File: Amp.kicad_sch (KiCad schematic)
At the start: 37 parts, among them J1 Screw_Terminal_01x02, J2 AudioJack2, J3 Screw_Terminal_01x02, J4 Screw_Terminal_01x02, J5 Screw_Terminal_01x02, P1 100k, U1 ECC83, U2 EL34, U3 EL34

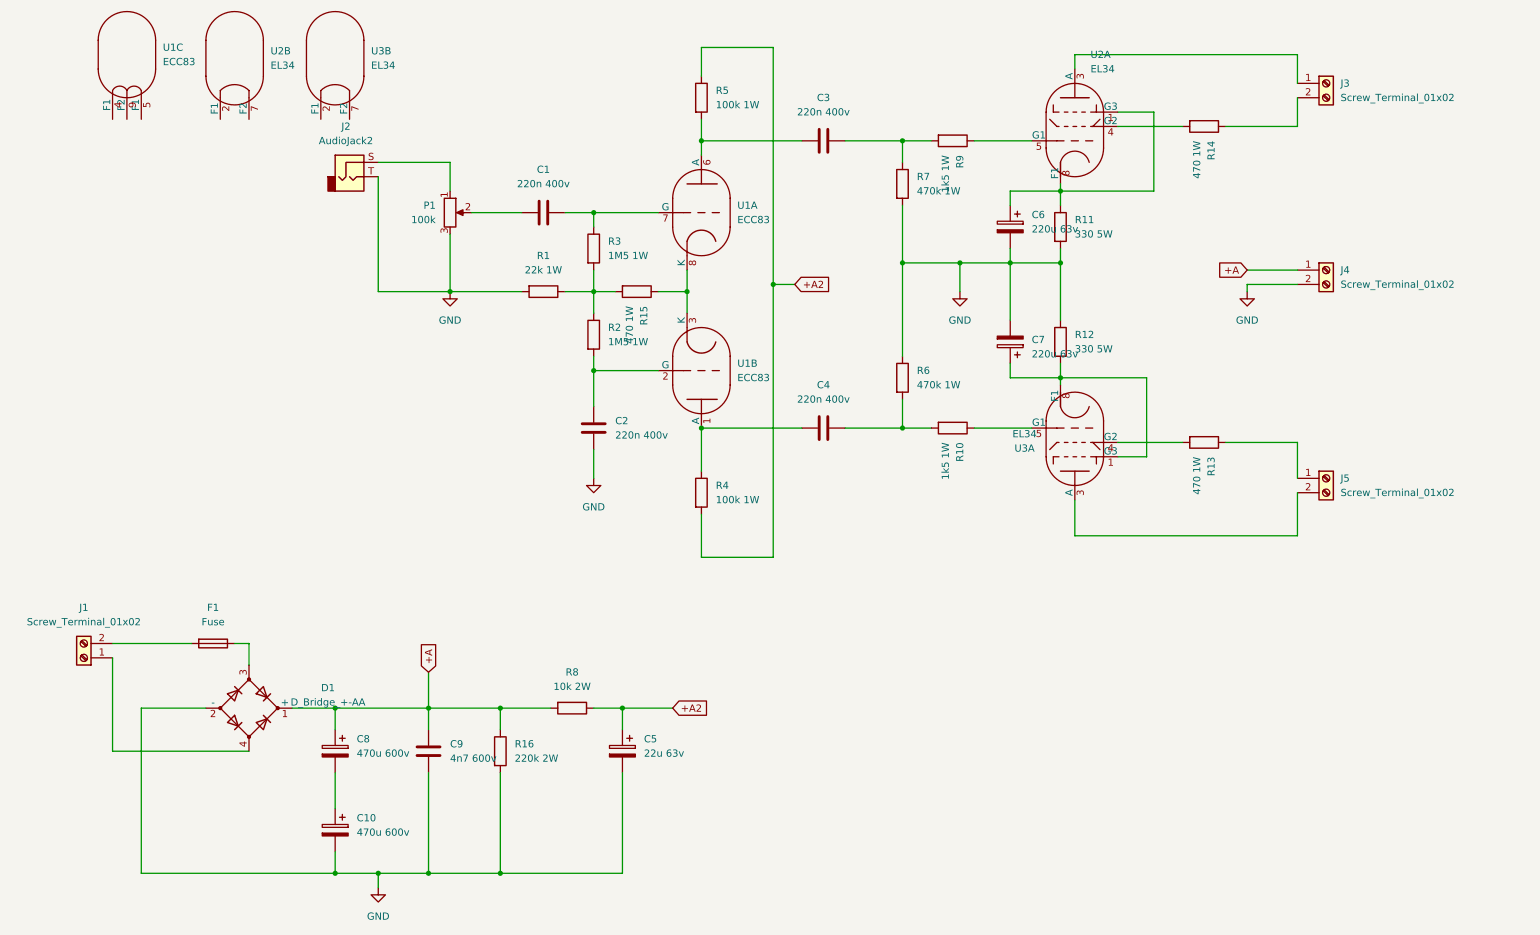
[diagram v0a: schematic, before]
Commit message: Update
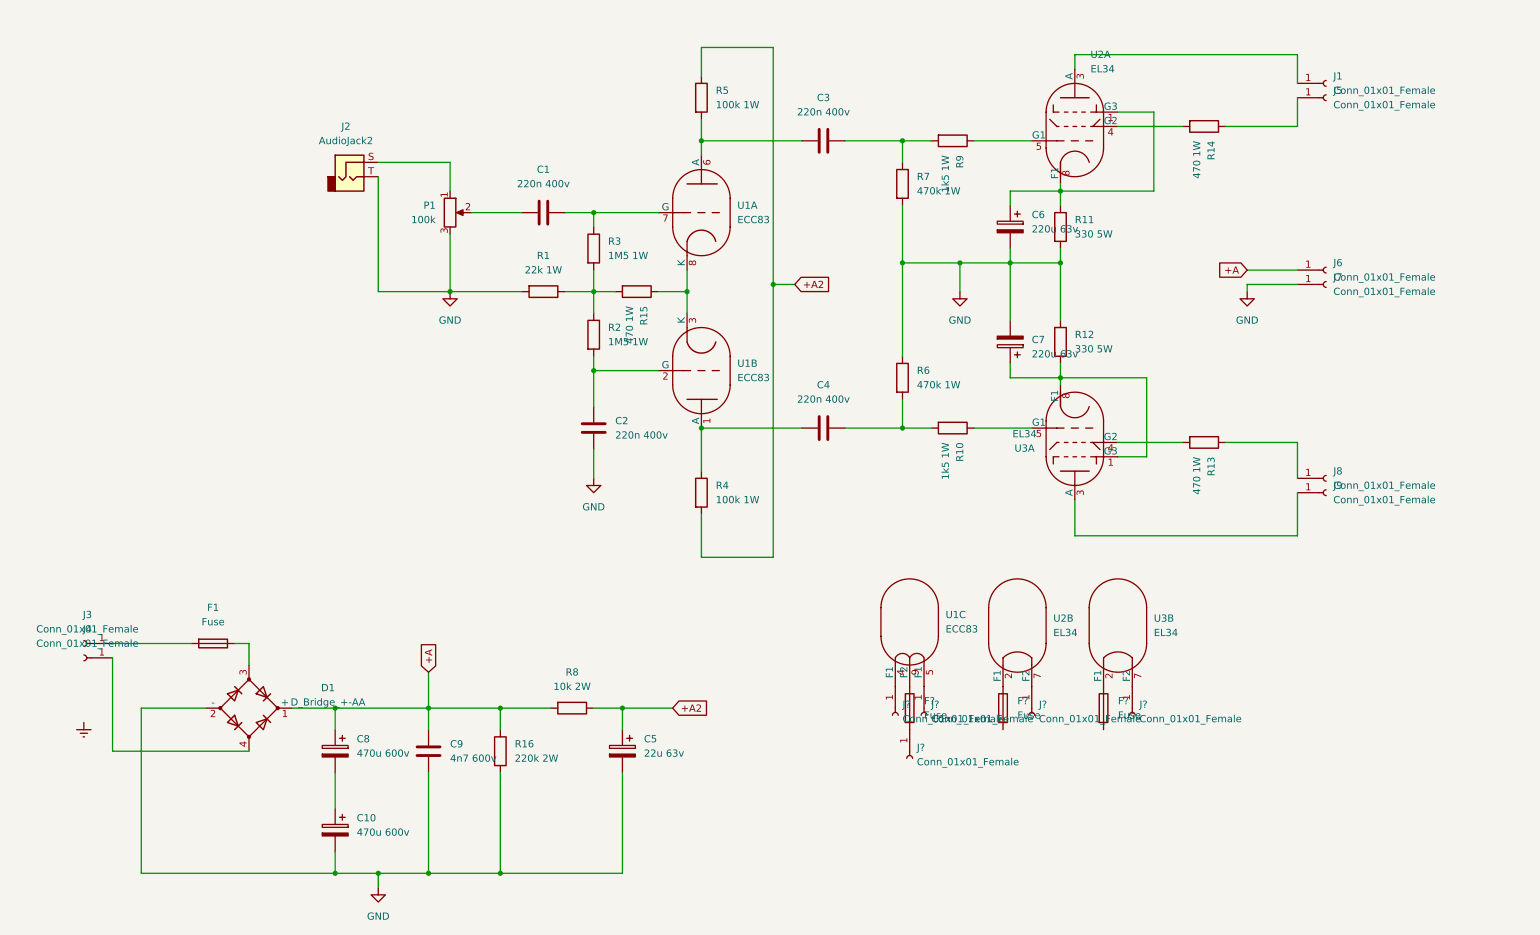
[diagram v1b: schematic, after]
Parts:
- removed J1, J3, J4, J5: Screw_Terminal_01x02, Connector:Banana_Jack_2Pin, symbol Connector:Screw_Terminal_01x02
- added F? (x3): Fuse, Fuse:Fuseholder_Cylinder-5x20mm_Schurter_0031_8201_Horizontal_Open, symbol Device:Fuse
- added J1, J3, J4, J5, J6, J7, J8, J9, J? (x5): Conn_01x01_Female, Connector_Pin:Pin_D1.0mm_L10.0mm, symbol Connector:Conn_01x01_Female
- F1: footprint (none) -> Fuse:Fuseholder_Cylinder-5x20mm_Schurter_0031_8201_Horizontal_Open
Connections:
- net +A: now also J6.1 (Pin_1)
- net GND: now also J7.1 (Pin_1)
- net at D1.4: now also J4.1 (Pin_1)
- net at F1.2: now also J3.1 (Pin_1)
- net at U1.4 (F1): now also J?.1 (Pin_1)
- net at U1.5 (F1): now also J?.1 (Pin_1)
- net at U1.9 (F2): now also F?.1
- net at R14.1: now also J5.1 (Pin_1)
- net at R13.1: now also J8.1 (Pin_1)
- net at U2.3 (A): now also J1.1 (Pin_1)
- net at U3.3 (A): now also J9.1 (Pin_1)
- net at U2.2 (F1): now also F?.1
- net at U2.7 (F2): now also J?.1 (Pin_1)
- net at U3.2 (F1): now also F?.1
- net at U3.7 (F2): now also J?.1 (Pin_1)
- new net: F?.2, J?.1 (Pin_1)
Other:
- moved on the sheet: U1C, U2B, U3B

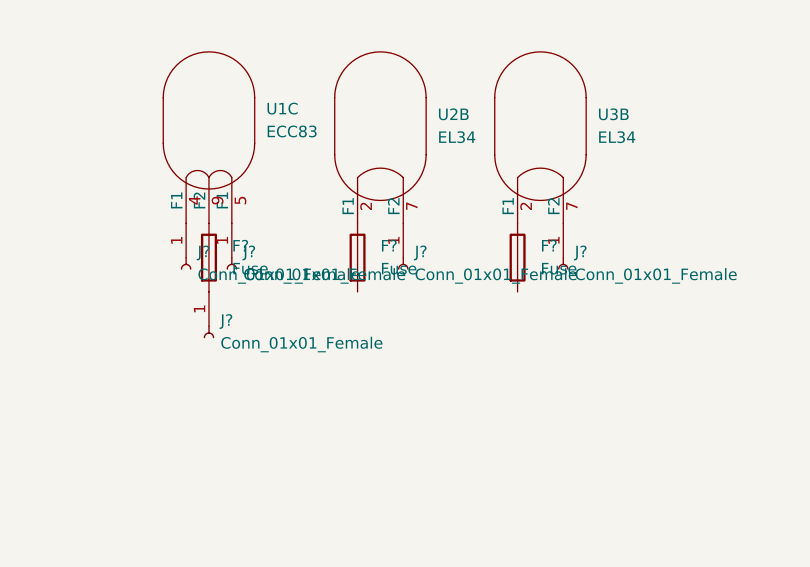
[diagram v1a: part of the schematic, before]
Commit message: Update
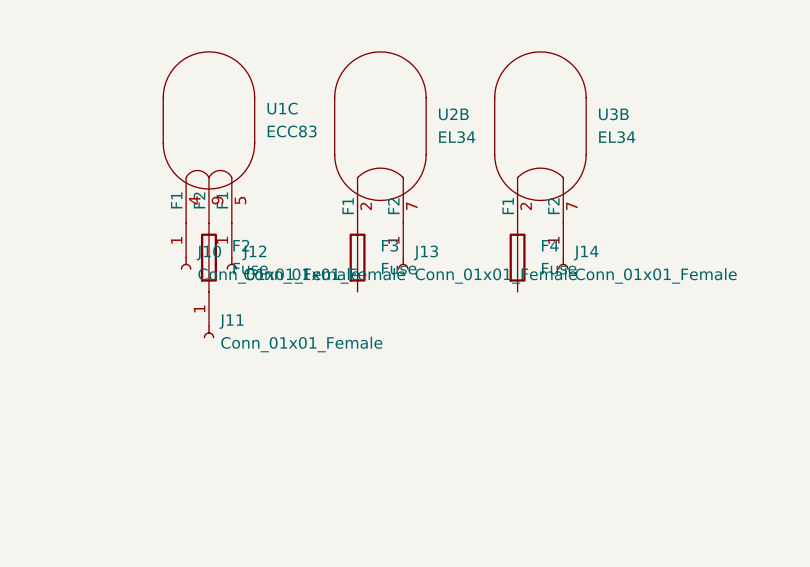
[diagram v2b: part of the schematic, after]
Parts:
- gave numbers to parts that had none: 8
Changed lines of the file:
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@@
   (symbol (lib_id "Device:Fuse") (at 186.69 139.7 0) (unit 1)
     (in_bom yes) (on_board yes) (fields_autoplaced)
-    (property "Reference" "F?" (id 0) (at 189.23 138.4299 0)
+    (property "Reference" "F3" (id 0) (at 189.23 138.4299 0)
       (effects (font (size 1.27 1.27)) (justify left))
     )
@@
   (symbol (lib_id "Device:Fuse") (at 204.47 139.7 0) (unit 1)
     (in_bom yes) (on_board yes) (fields_autoplaced)
-    (property "Reference" "F?" (id 0) (at 207.01 138.4299 0)
+    (property "Reference" "F4" (id 0) (at 207.01 138.4299 0)
       (effects (font (size 1.27 1.27)) (justify left))
     )
@@
   (symbol (lib_id "Connector:Conn_01x01_Female") (at 170.18 148.59 270) (unit 1)
     (in_bom yes) (on_board yes) (fields_autoplaced)
-    (property "Reference" "J?" (id 0) (at 171.45 146.6849 90)
+    (property "Reference" "J11" (id 0) (at 171.45 146.6849 90)
       (effects (font (size 1.27 1.27)) (justify left))
     )
@@
   (symbol (lib_id "Device:Fuse") (at 170.18 139.7 0) (unit 1)
     (in_bom yes) (on_board yes) (fields_autoplaced)
-    (property "Reference" "F?" (id 0) (at 172.72 138.4299 0)
+    (property "Reference" "F2" (id 0) (at 172.72 138.4299 0)
       (effects (font (size 1.27 1.27)) (justify left))
     )
@@
   (symbol (lib_id "Connector:Conn_01x01_Female") (at 167.64 140.97 270) (unit 1)
     (in_bom yes) (on_board yes) (fields_autoplaced)
-    (property "Reference" "J?" (id 0) (at 168.91 139.0649 90)
+    (property "Reference" "J10" (id 0) (at 168.91 139.0649 90)
       (effects (font (size 1.27 1.27)) (justify left))
     )
@@
   (symbol (lib_id "Connector:Conn_01x01_Female") (at 209.55 140.97 270) (unit 1)
     (in_bom yes) (on_board yes) (fields_autoplaced)
-    (property "Reference" "J?" (id 0) (at 210.82 139.0649 90)
+    (property "Reference" "J14" (id 0) (at 210.82 139.0649 90)
       (effects (font (size 1.27 1.27)) (justify left))
     )
@@
   (symbol (lib_id "Connector:Conn_01x01_Female") (at 191.77 140.97 270) (unit 1)
     (in_bom yes) (on_board yes) (fields_autoplaced)
-    (property "Reference" "J?" (id 0) (at 193.04 139.0649 90)
+    (property "Reference" "J13" (id 0) (at 193.04 139.0649 90)
       (effects (font (size 1.27 1.27)) (justify left))
     )
@@
   (symbol (lib_id "Connector:Conn_01x01_Female") (at 172.72 140.97 270) (unit 1)
     (in_bom yes) (on_board yes) (fields_autoplaced)
-    (property "Reference" "J?" (id 0) (at 173.99 139.0649 90)
+    (property "Reference" "J12" (id 0) (at 173.99 139.0649 90)
       (effects (font (size 1.27 1.27)) (justify left))
     )
@@
       (reference "F1") (unit 1) (value "Fuse") (footprint "Fuse:Fuseholder_Cylinder-5x20mm_Schurter_0031_8201_Horizontal_Open")
     )
+    (path "/a1adcb6c-db44-4b49-93cb-68ae942fb387"
+      (reference "F2") (unit 1) (value "Fuse") (footprint "Fuse:Fuseholder_Cylinder-5x20mm_Schurter_0031_8201_Horizontal_Open")
+    )
     (path "/25fbb172-8ec9-4c95-8bc3-97f4ffc44970"
-      (reference "F?") (unit 1) (value "Fuse") (footprint "Fuse:Fuseholder_Cylinder-5x20mm_Schurter_0031_8201_Horizontal_Open")
+      (reference "F3") (unit 1) (value "Fuse") (footprint "Fuse:Fuseholder_Cylinder-5x20mm_Schurter_0031_8201_Horizontal_Open")
     )
     (path "/6e05b8a2-376d-4b46-b83d-ba7e6ff52c0c"
-      (reference "F?") (unit 1) (value "Fuse") (footprint "Fuse:Fuseholder_Cylinder-5x20mm_Schurter_0031_8201_Horizontal_Open")
-    )
-    (path "/a1adcb6c-db44-4b49-93cb-68ae942fb387"
-      (reference "F?") (unit 1) (value "Fuse") (footprint "Fuse:Fuseholder_Cylinder-5x20mm_Schurter_0031_8201_Horizontal_Open")
+      (reference "F4") (unit 1) (value "Fuse") (footprint "Fuse:Fuseholder_Cylinder-5x20mm_Schurter_0031_8201_Horizontal_Open")
     )
     (path "/61c97752-6da3-4341-ab98-f5445eac9c73"
@@
       (reference "J9") (unit 1) (value "Conn_01x01_Female") (footprint "Connector_Pin:Pin_D1.0mm_L10.0mm")
     )
+    (path "/b5815324-6ba2-42f0-9780-104e90daf288"
+      (reference "J10") (unit 1) (value "Conn_01x01_Female") (footprint "Connector_Pin:Pin_D1.0mm_L10.0mm")
+    )
     (path "/72a3e0c6-7ea5-445a-8b6e-f4f233fb6743"
-      (reference "J?") (unit 1) (value "Conn_01x01_Female") (footprint "Connector_Pin:Pin_D1.0mm_L10.0mm")
-    )
-    (path "/b5815324-6ba2-42f0-9780-104e90daf288"
-      (reference "J?") (unit 1) (value "Conn_01x01_Female") (footprint "Connector_Pin:Pin_D1.0mm_L10.0mm")
+      (reference "J11") (unit 1) (value "Conn_01x01_Female") (footprint "Connector_Pin:Pin_D1.0mm_L10.0mm")
+    )
+    (path "/f0993887-d724-43e0-a22c-a1c622282bd8"
+      (reference "J12") (unit 1) (value "Conn_01x01_Female") (footprint "Connector_Pin:Pin_D1.0mm_L10.0mm")
+    )
+    (path "/e48ab2ba-f66f-4a03-9892-4352a1c7ac9f"
+      (reference "J13") (unit 1) (value "Conn_01x01_Female") (footprint "Connector_Pin:Pin_D1.0mm_L10.0mm")
     )
     (path "/b6988044-dd27-4444-9c1d-a6a06e5158f8"
-      (reference "J?") (unit 1) (value "Conn_01x01_Female") (footprint "Connector_Pin:Pin_D1.0mm_L10.0mm")
-    )
-    (path "/e48ab2ba-f66f-4a03-9892-4352a1c7ac9f"
-      (reference "J?") (unit 1) (value "Conn_01x01_Female") (footprint "Connector_Pin:Pin_D1.0mm_L10.0mm")
-    )
-    (path "/f0993887-d724-43e0-a22c-a1c622282bd8"
-      (reference "J?") (unit 1) (value "Conn_01x01_Female") (footprint "Connector_Pin:Pin_D1.0mm_L10.0mm")
+      (reference "J14") (unit 1) (value "Conn_01x01_Female") (footprint "Connector_Pin:Pin_D1.0mm_L10.0mm")
     )
     (path "/83260ffb-4f0b-4387-910e-aee74b14be4e"

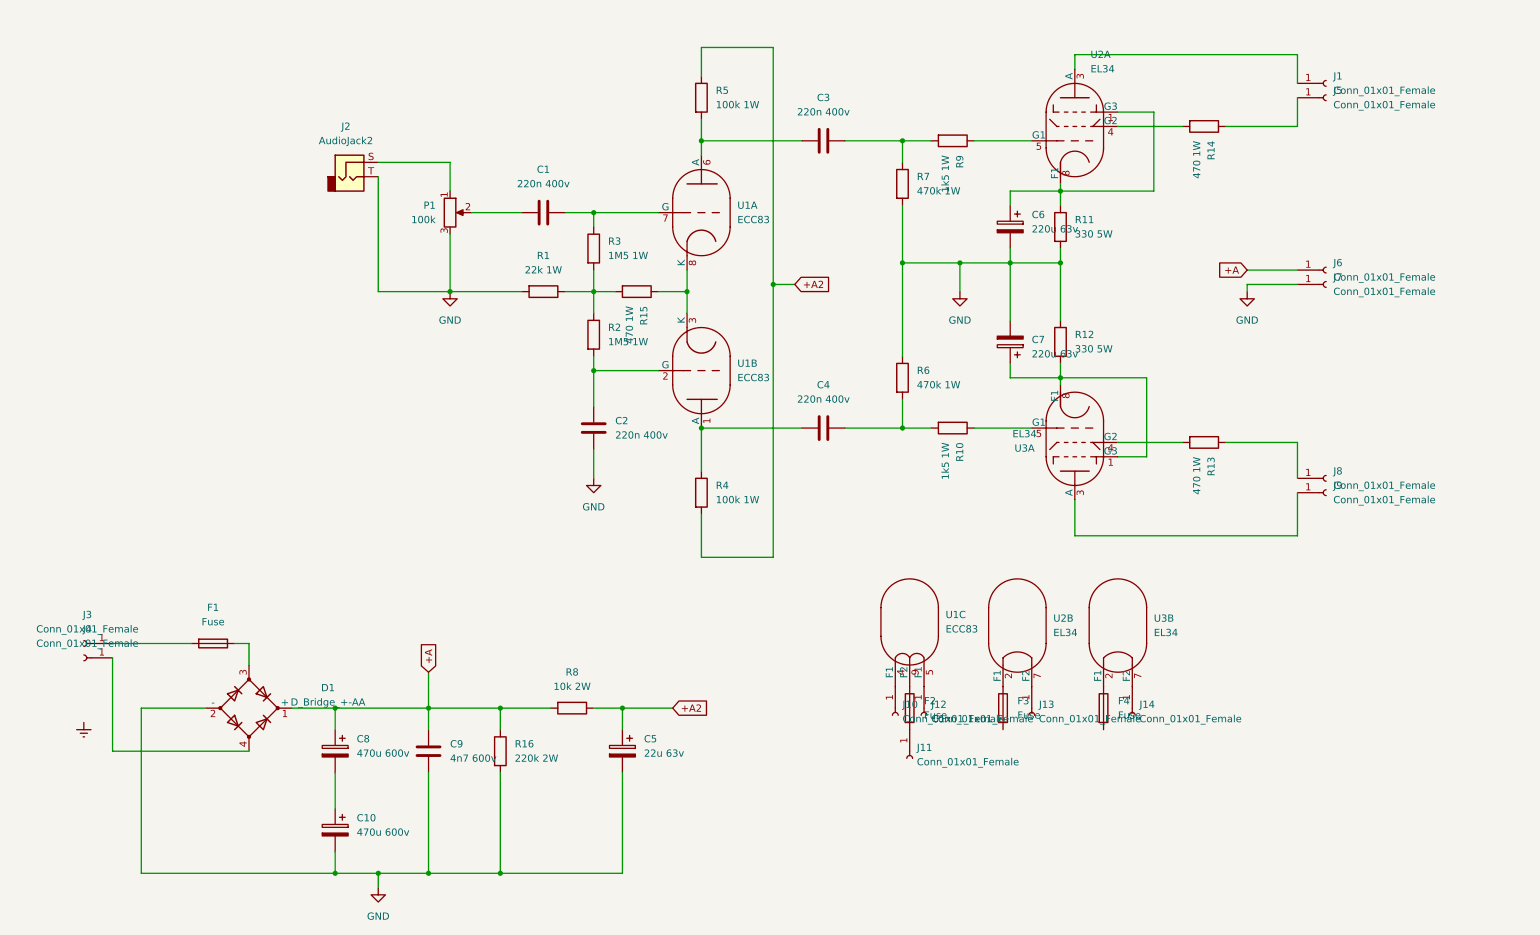
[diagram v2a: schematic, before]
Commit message: Update, cleanup
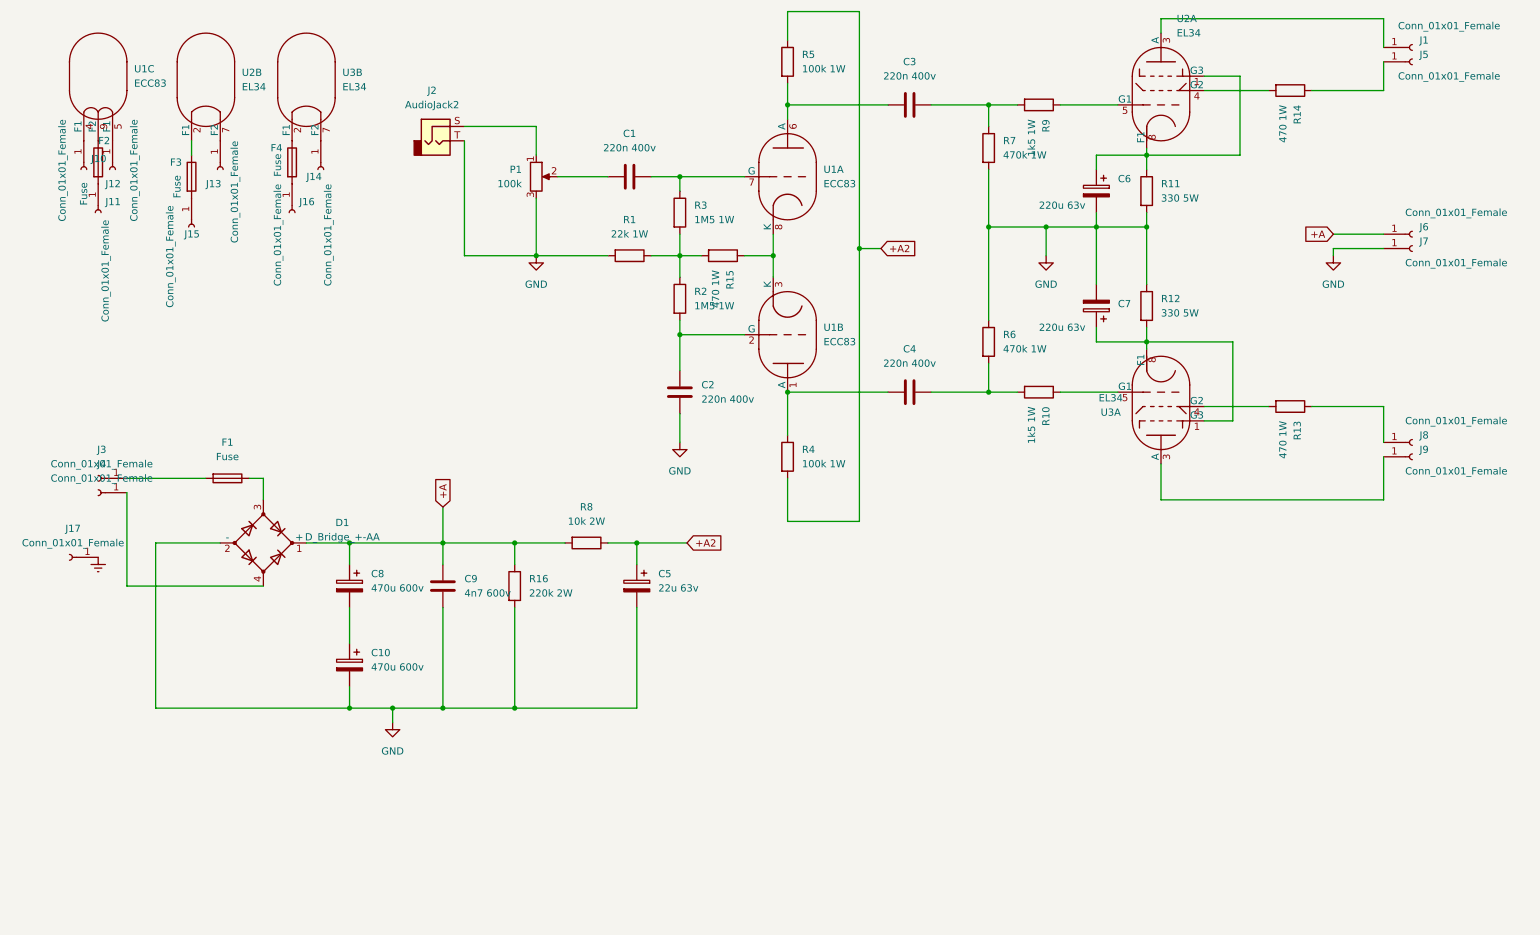
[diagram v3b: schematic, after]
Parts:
- added J15, J16, J17: Conn_01x01_Female, Connector_Pin:Pin_D1.0mm_L10.0mm, symbol Connector:Conn_01x01_Female
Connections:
- net Earth: now also J17.1 (Pin_1)
- net at F3.2: now also J15.1 (Pin_1)
- net at F4.2: now also J16.1 (Pin_1)
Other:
- moved on the sheet: C1, C10, C2, C3, C4, C5, C6, C7, C8, C9, D1, F1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
